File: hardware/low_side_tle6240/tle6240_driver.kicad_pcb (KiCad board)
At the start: 2 copper layers, 58.4 x 50.8 mm, 17 parts, among them K1 CONN_3, P1 CONN_10X2, P2 CONN_2, P3 CONN_4, P4 CONN_4, P5 CONN_4, P6 CONN_4

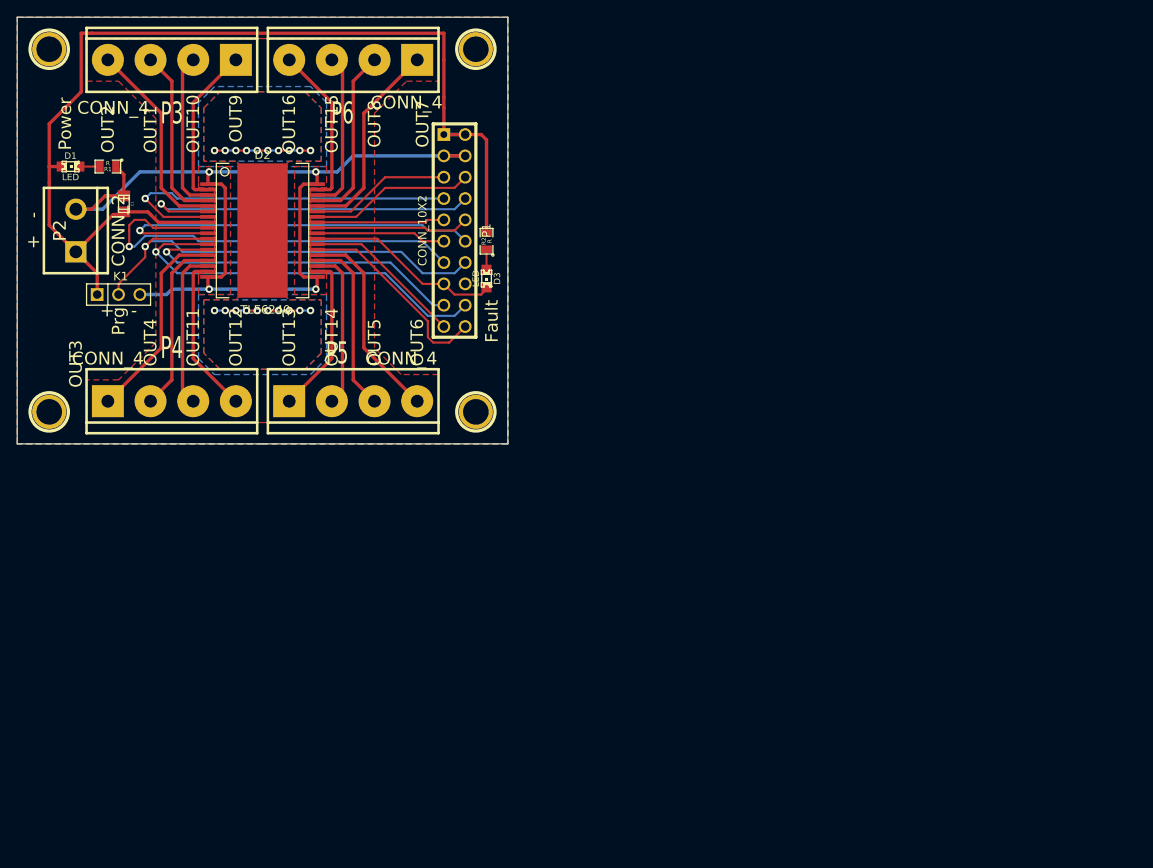
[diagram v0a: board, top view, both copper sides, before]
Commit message: v2
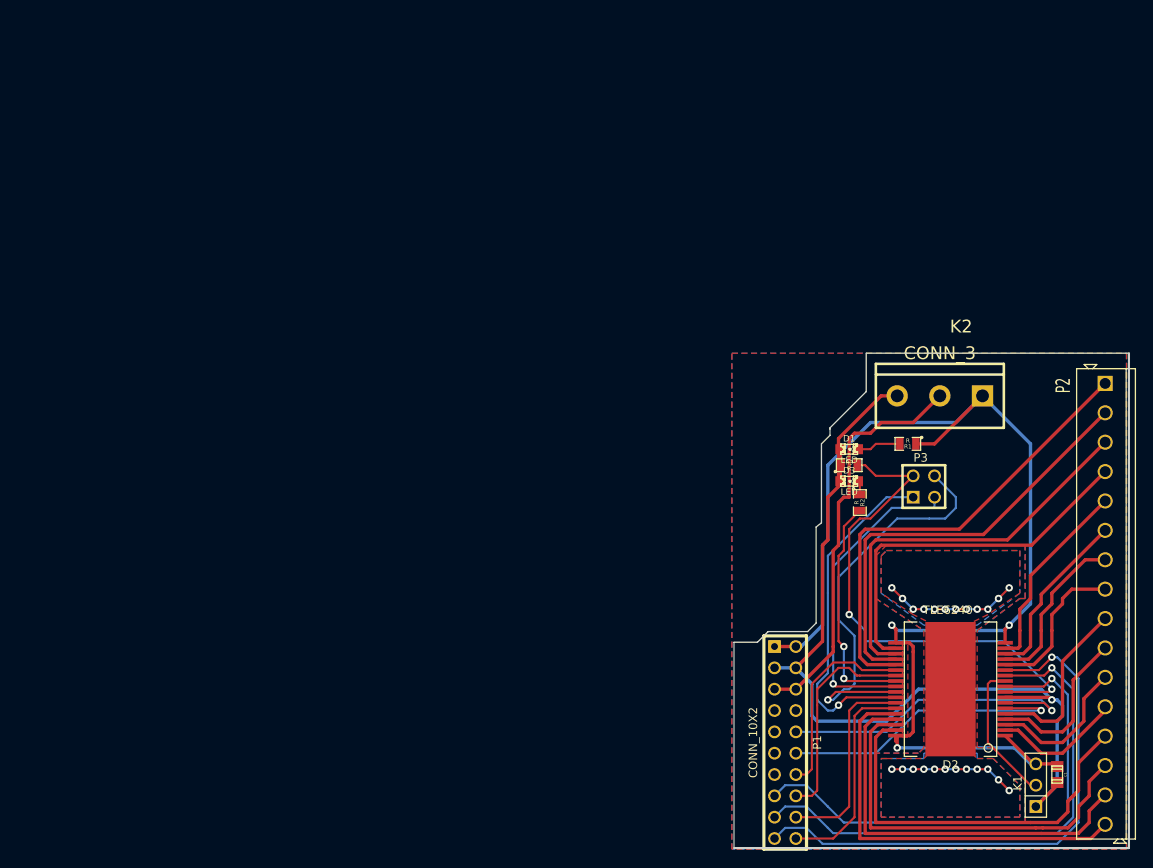
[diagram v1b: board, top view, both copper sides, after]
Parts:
- removed ? (x4): , 1pin
- removed P4, P5, P6: CONN_4, bornier4
- added K2: CONN_3, bornier3, F.Cu at (197.5, 97.2)
- added R3: R, SM0805, F.Cu at (186.7, 105.4)
- P2: value CONN_2 -> CONN_16; footprint bornier2 -> SIL-16_3.5MM
- P3: value CONN_4 -> CONN_2X2; footprint bornier4 -> PIN_ARRAY_2X2
- moved P2 130.4 mm to (217.2, 121.9), turned to 270 degrees
- moved C1 130.3 mm to (211.5, 142.2)
- moved K1 123.9 mm to (208.9, 143.5), turned to 90 degrees
- moved P3 102.9 mm to (195.6, 108.0), turned to 0 degrees
- moved R1 100.8 mm to (193.7, 102.9)
- moved D1 98.6 mm to (186.7, 103.5)
- moved D2 98.4 mm to (198.8, 132.1), turned to 180 degrees
- moved P1 72.6 mm to (179.1, 138.4)
- moved R2 54.3 mm to (188.0, 109.9), turned to 270 degrees
- moved D3 49.5 mm to (186.7, 107.3), turned to 0 degrees
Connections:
- D3 pad 1: N-0000034 -> +5V
- D3 pad 2: /Fault -> N-0000015
- P1 pad 1: +5V -> GND
- P1 pad 10: /SCLK -> /IN2
- P1 pad 11: /SO -> (no net)
- P1 pad 12: /CS -> /IN1
- P1 pad 13: /Reset -> (no net)
- P1 pad 14: /PRG -> /IN9
- P1 pad 15: /Fault -> /CS
- P1 pad 16: (no net) -> /IN10
- P1 pad 17: /IN4 -> /IN3
- P1 pad 18: /IN3 -> /IN11
- P1 pad 19: /IN10 -> /IN4
- P1 pad 2: +5V -> GND
- P1 pad 20: /IN9 -> /IN12
- P1 pad 3: GND -> +5V
- P1 pad 4: GND -> +5V
- P1 pad 5: /IN12 -> /+3.3V
- P1 pad 6: /IN11 -> /+3.3V
- P1 pad 7: /IN2 -> (no net)
- P1 pad 8: /IN1 -> (no net)
- P1 pad 9: /SI -> (no net)
- P2 pad 1: +5V -> /OUT6
- P2 pad 2: GND -> /OUT5
- P3 pad 1: /OUT9 -> /SI
- P3 pad 2: /OUT10 -> /Reset
- P3 pad 3: /OUT1 -> /SO
- P3 pad 4: /OUT2 -> /SCLK
- R2 pad 1: N-0000034 -> N-0000015
- R2 pad 2: +5V -> /Fault
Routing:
- net /+3.3V: track 0.00 -> 48.3 mm
- net /PRG: track 55.4 -> 17.0 mm, vias 1 -> 0
- net GND: track 118.4 -> 150.6 mm, vias 4 -> 3
- net /OUT6: track 24.3 -> 55.9 mm
- net /OUT5: track 21.2 -> 52.2 mm
- net /SCLK: track 18.3 -> 48.2 mm, vias 0 -> 1
- net /OUT16: track 19.2 -> 49.0 mm
- net /OUT14: track 19.1 -> 48.5 mm
- net /OUT15: track 19.1 -> 47.6 mm
- net /OUT8: track 21.2 -> 48.0 mm
- net /SI: track 15.2 -> 41.3 mm, vias 0 -> 1
- net /OUT13: track 19.2 -> 44.7 mm
- net /IN4: track 40.7 -> 66.1 mm
- net /OUT7: track 24.3 -> 48.5 mm
- net /SO: track 15.5 -> 37.8 mm, vias 0 -> 1
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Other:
- board size 58.4 x 50.8 mm -> 47 x 58.9 mm
- net class Power added: clearance 0.154, trace_width 0.4, via_dia 0.889, via_drill 0.635
- net class power removed
- board text removed: "+ -"
- board text removed: "Fault"
- board text removed: "OUT1"
- board text removed: "OUT10"
- board text removed: "OUT11"
- board text removed: "OUT12"
- board text removed: "OUT13"
- board text removed: "OUT14"
- board text removed: "OUT15"
- board text removed: "OUT16"
- board text removed: "OUT2"
- board text removed: "OUT3"
- board text removed: "OUT4"
- board text removed: "OUT5"
- board text removed: "OUT6"
- board text removed: "OUT7"
- board text removed: "OUT8"
- board text removed: "OUT9"
- board text removed: "Power"
- board text removed: "Prg"
